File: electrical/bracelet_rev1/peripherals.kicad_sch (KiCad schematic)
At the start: 4 parts, among them U2 LSM6DSO32TR

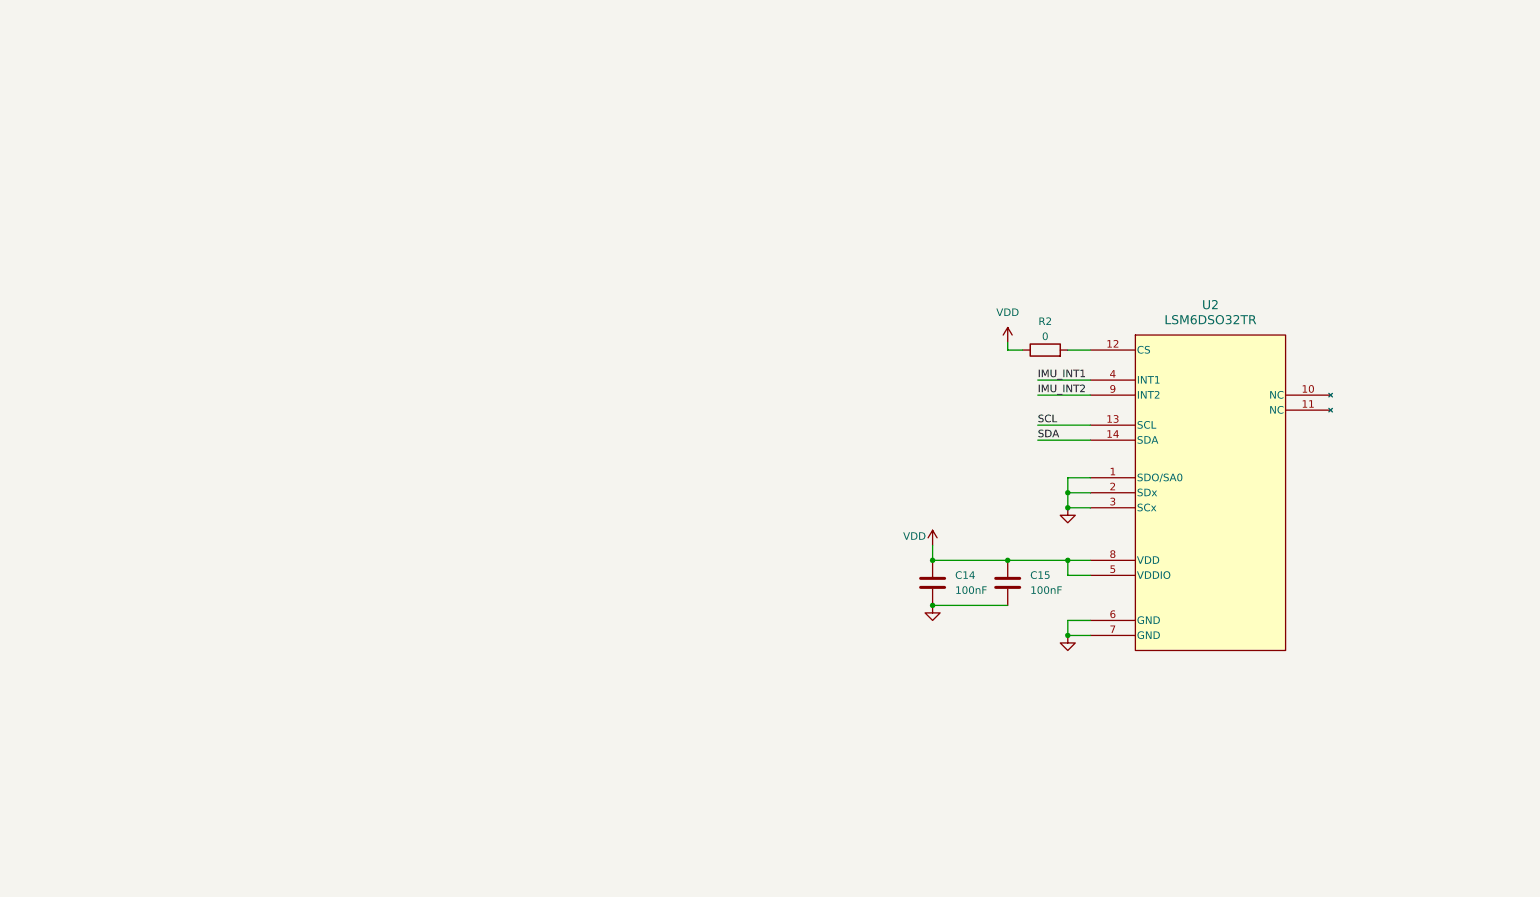
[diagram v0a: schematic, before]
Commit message: Many schematic updates
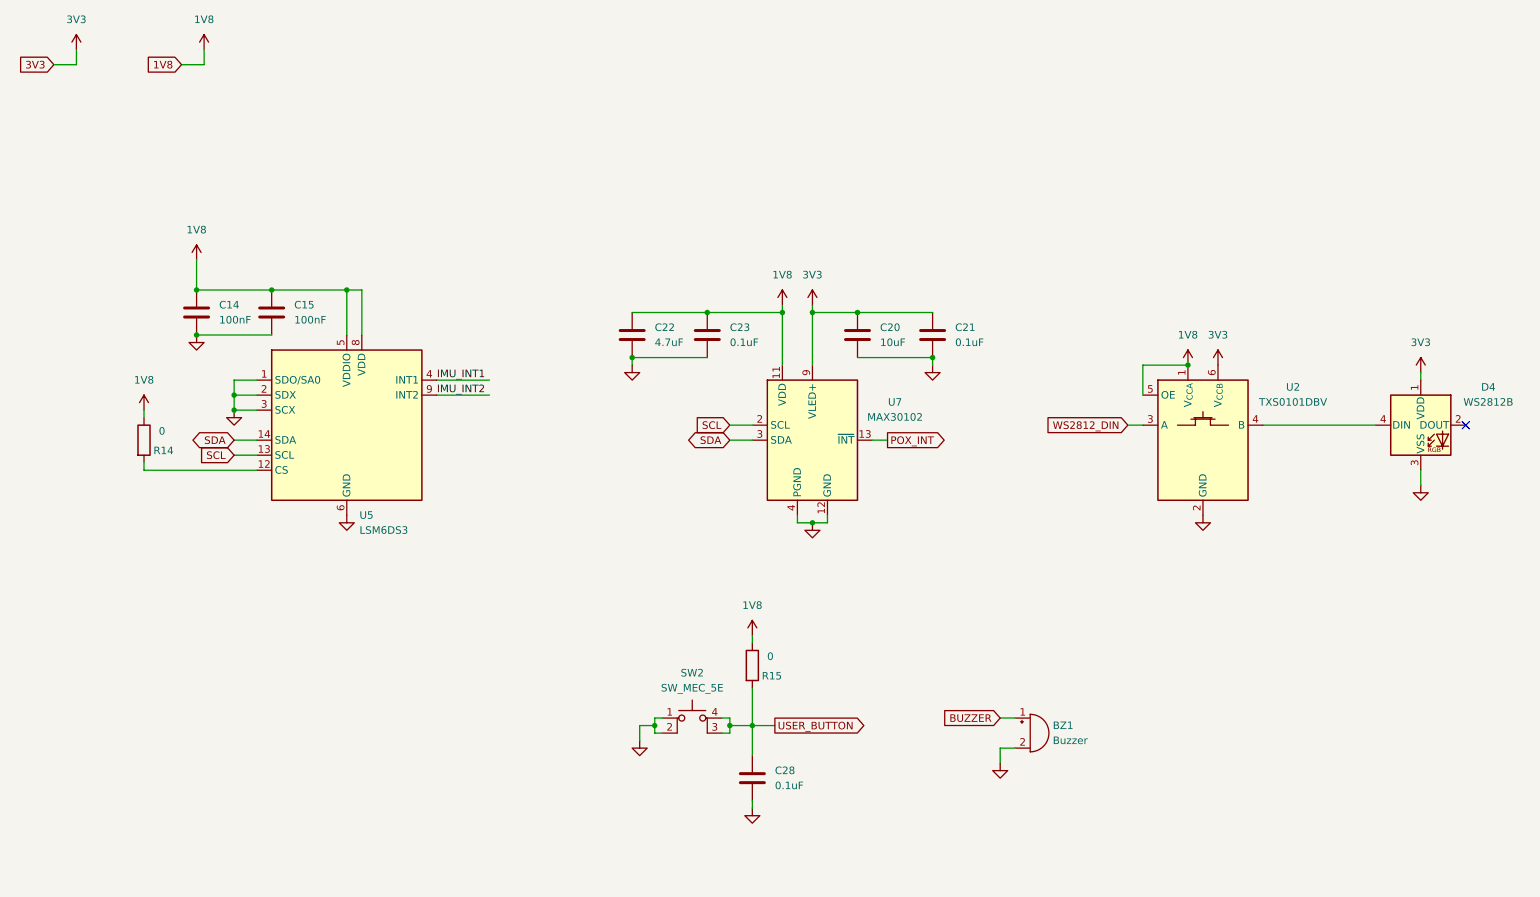
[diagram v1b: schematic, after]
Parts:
- removed R2: 0, symbol Device:R
- removed U2: LSM6DSO32TR, LGA-14L_2P5X3X0P83_STM, symbol IMU:LSM6DSO32TR
- added BZ1: Buzzer, symbol Device:Buzzer
- added C20: 10uF, symbol Device:C
- added C21, C23, C28: 0.1uF, symbol Device:C
- added C22: 4.7uF, symbol Device:C
- added D4: WS2812B, LED_SMD:LED_WS2812B_PLCC4_5.0x5.0mm_P3.2mm, symbol LED:WS2812B
- added R14, R15: 0, symbol Device:R
- added SW2: SW_MEC_5E, symbol Switch:SW_MEC_5E
- added U2: TXS0101DBV, Package_TO_SOT_SMD:SOT-23-6, symbol Logic_LevelTranslator:TXS0101DBV
- added U5: LSM6DS3, Package_LGA:LGA-14_3x2.5mm_P0.5mm_LayoutBorder3x4y, symbol Sensor_Motion:LSM6DS3
- added U7: MAX30102, OptoDevice:Maxim_OLGA-14_3.3x5.6mm_P0.8mm, symbol Sensor:MAX30102
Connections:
- net GND: now also BZ1.2 (-), C20.2, C21.2, C22.2, C23.2, C28.2, D4.3 (VSS), SW2.1, SW2.2, U2.2 (GND), U5.1 (SDO/SA0), U5.2 (SDX), U5.3 (SCX), U5.6 (GND), U5.7 (GND), U7.12 (GND), U7.4 (PGND)
- net IMU_INT1: now also U5.4 (INT1)
- net IMU_INT2: now also U5.9 (INT2)
- net SCL: now also U5.13 (SCL), U7.2 (SCL)
- net SDA: now also U5.14 (SDA), U7.3 (SDA)
- net VDD renamed 1V8
- net 1V8: now also C22.1, C23.1, R14.1, R15.1, U2.1 (V_{CCA}), U2.5 (OE), U5.5 (VDDIO), U5.8 (VDD), U7.11 (VDD)
- new net: D4.4 (DIN), U2.4 (B)
- new net: R14.2, U5.12 (CS)
- new net 3V3: C20.1, C21.1, D4.1 (VDD), U2.6 (V_{CCB}), U7.10 (VLED+), U7.9 (VLED+)
- new net BUZZER: BZ1.1 (+)
- new net POX_INT: U7.13 (~{INT})
- new net USER_BUTTON: C28.1, R15.2, SW2.3 (K), SW2.4 (A)
- new net WS2812_DIN: U2.3 (A)
- no-connect marks 0 -> 1
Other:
- moved on the sheet: C14, C15

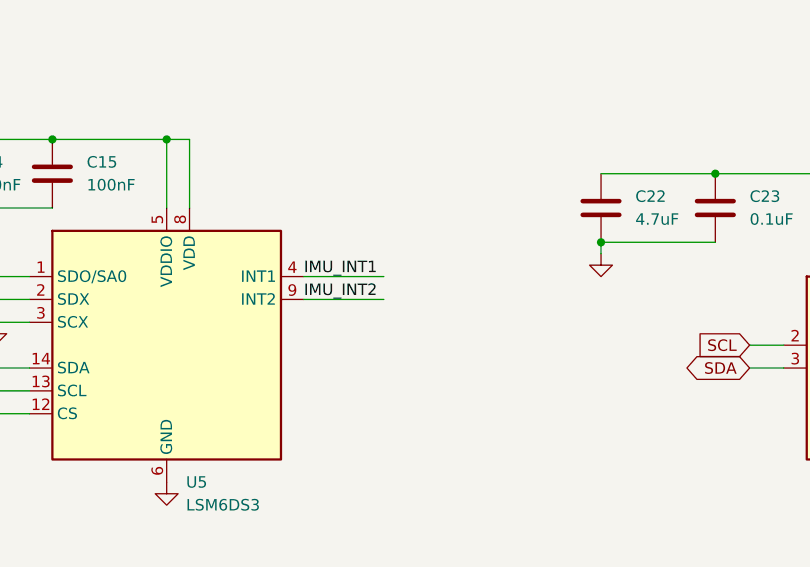
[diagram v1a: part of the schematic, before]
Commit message: Mostly finihsed hopefully but still needs clean up anyway
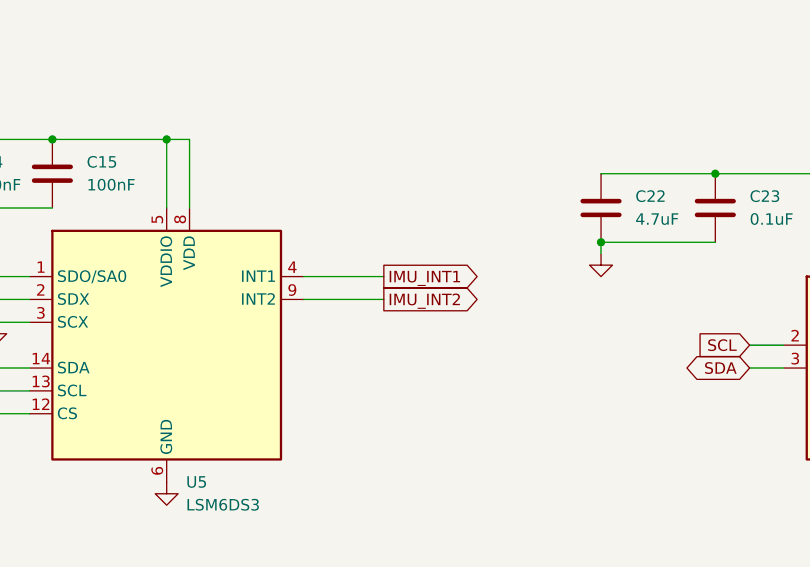
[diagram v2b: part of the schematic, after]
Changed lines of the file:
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@@
-		)
-	)
-	(label "IMU_INT2"
-		(at 90.17 81.28 0)
-		(effects
-			(font
-				(size 1.27 1.27)
-			)
-			(justify left bottom)
-		)
-	)
-	(label "IMU_INT1"
-		(at 90.17 78.74 0)
-		(effects
-			(font
-				(size 1.27 1.27)
-			)
-			(justify left bottom)
 		)
 	)
@@
 		)
 	)
+	(global_label "IMU_INT2"
+		(shape output)
+		(at 99.06 81.28 0)
+		(fields_autoplaced yes)
+		(effects
+			(font
+				(size 1.27 1.27)
+			)
+			(justify left)
+		)
+		(property "Intersheetrefs" "${INTERSHEET_REFS}"
+			(at 110.5119 81.28 0)
+			(effects
+				(font
+					(size 1.27 1.27)
+				)
+				(justify left)
+				(hide yes)
+			)
+		)
+	)
 	(global_label "BUZZER"
 		(shape input)
@@
 				(hide yes)
 			)
+		)
+	)
+	(global_label "IMU_INT1"
+		(shape output)
+		(at 99.06 78.74 0)
+		(fields_autoplaced yes)
+		(effects
+			(font
+				(size 1.27 1.27)
+			)
+			(justify left)
+		)
+		(property "Intersheetrefs" "${INTERSHEET_REFS}"
+			(at 110.5119 78.74 0)
+			(effects
+				(font
+					(size 1.27 1.27)
+				)
+				(justify left)
+				(hide yes)
+			)

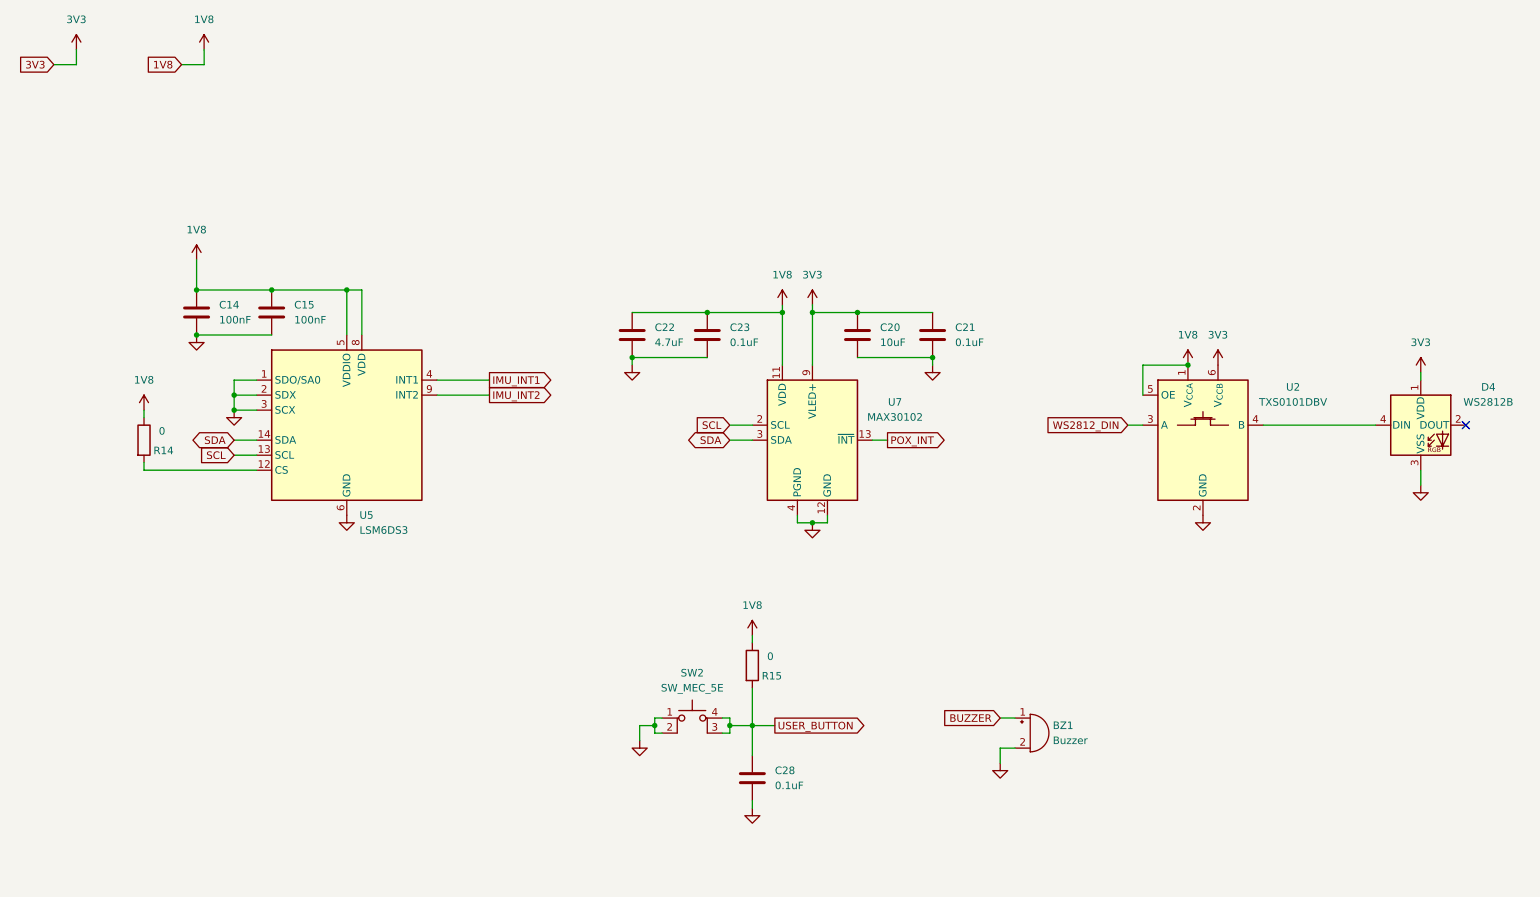
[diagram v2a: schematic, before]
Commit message: May updates
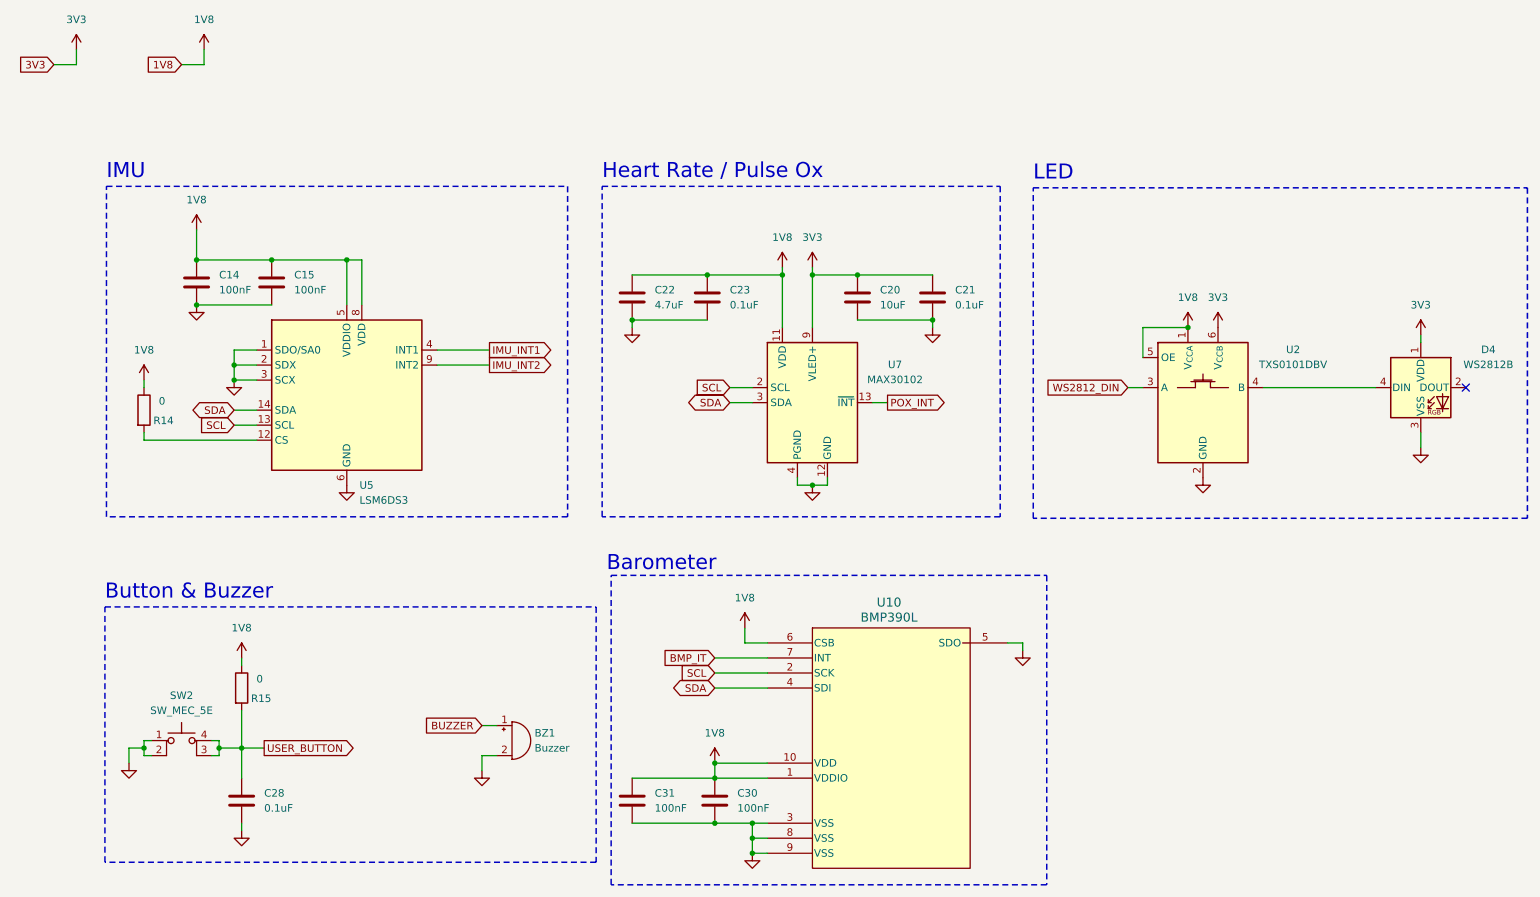
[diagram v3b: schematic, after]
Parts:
- added C30, C31: 100nF, symbol Device:C
- added U10: BMP390L, 10LGA_2X2X0p75_BOS, symbol Barometer:BMP390L
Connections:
- net 1V8: now also C30.1, C31.1, U10.1 (VDDIO), U10.10 (VDD), U10.6 (CSB)
- net GND: now also C30.2, C31.2, U10.3 (VSS), U10.5 (SDO), U10.8 (VSS), U10.9 (VSS)
- net SCL: now also U10.2 (SCK)
- net SDA: now also U10.4 (SDI)
- new net BMP_IT: U10.7 (INT)
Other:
- note added: "Barometer"
- note added: "Button & Buzzer"
- note added: "Heart Rate / Pulse Ox"
- note added: "IMU"
- note added: "LED"
- moved on the sheet: BZ1, C14, C15, C20, C21, C22, C23, C28, D4, R14, R15, SW2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
